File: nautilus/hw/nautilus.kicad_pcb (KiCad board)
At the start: 4 copper layers, 54.8 x 54 mm, 107 parts, among them IC1 DRV8353SRTAR, IC2 STM32G474CEU6, IC3 MAX15062AATA+T, J1 XT30XT30PW_MALE, J2 Conn_01x02_Pin, J3 Conn_01x02_Pin, M1 PAD24AWG_PAD, M2 PAD24AWG_PAD, M3 PAD24AWG_PAD, U2 CSD88599Q5DCT, U3 CSD88599Q5DCT, U4 AS5147, U5 CSD88599Q5DCT

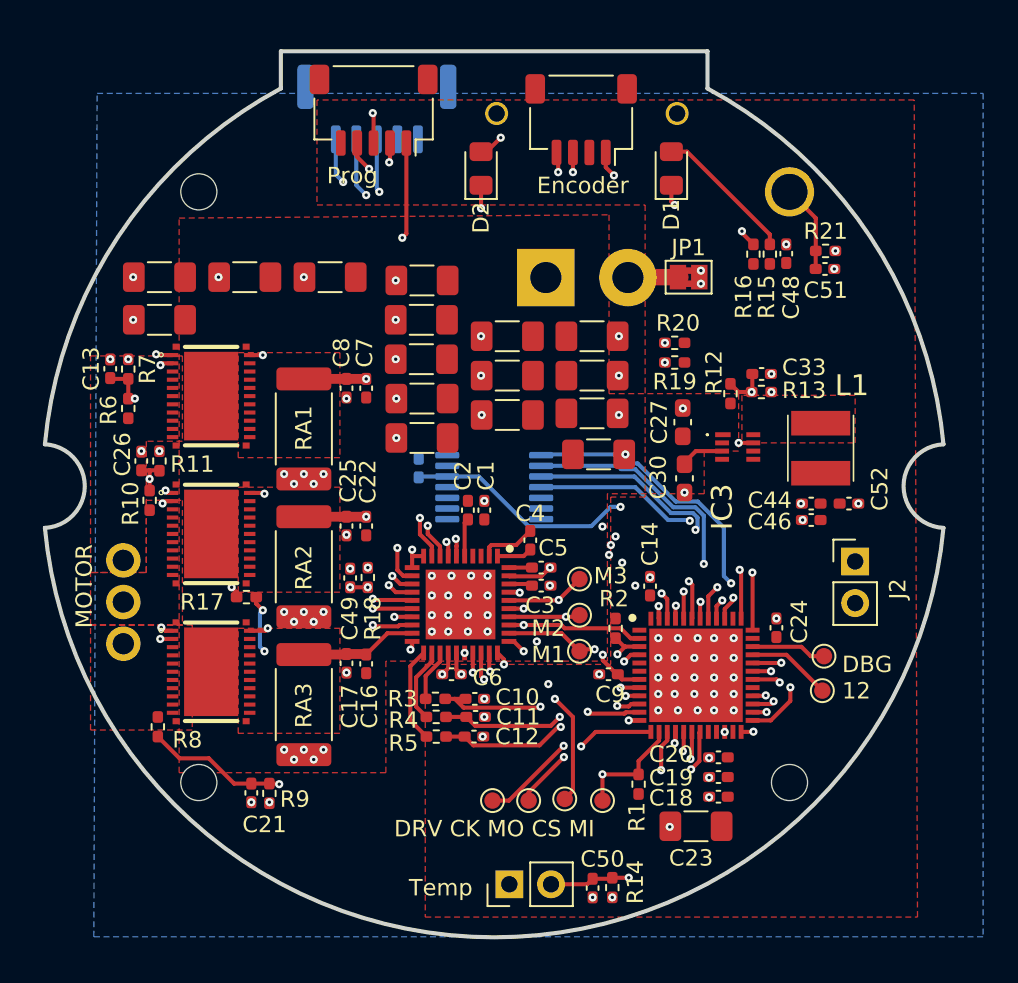
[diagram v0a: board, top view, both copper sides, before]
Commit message: Cleanup PCB before order
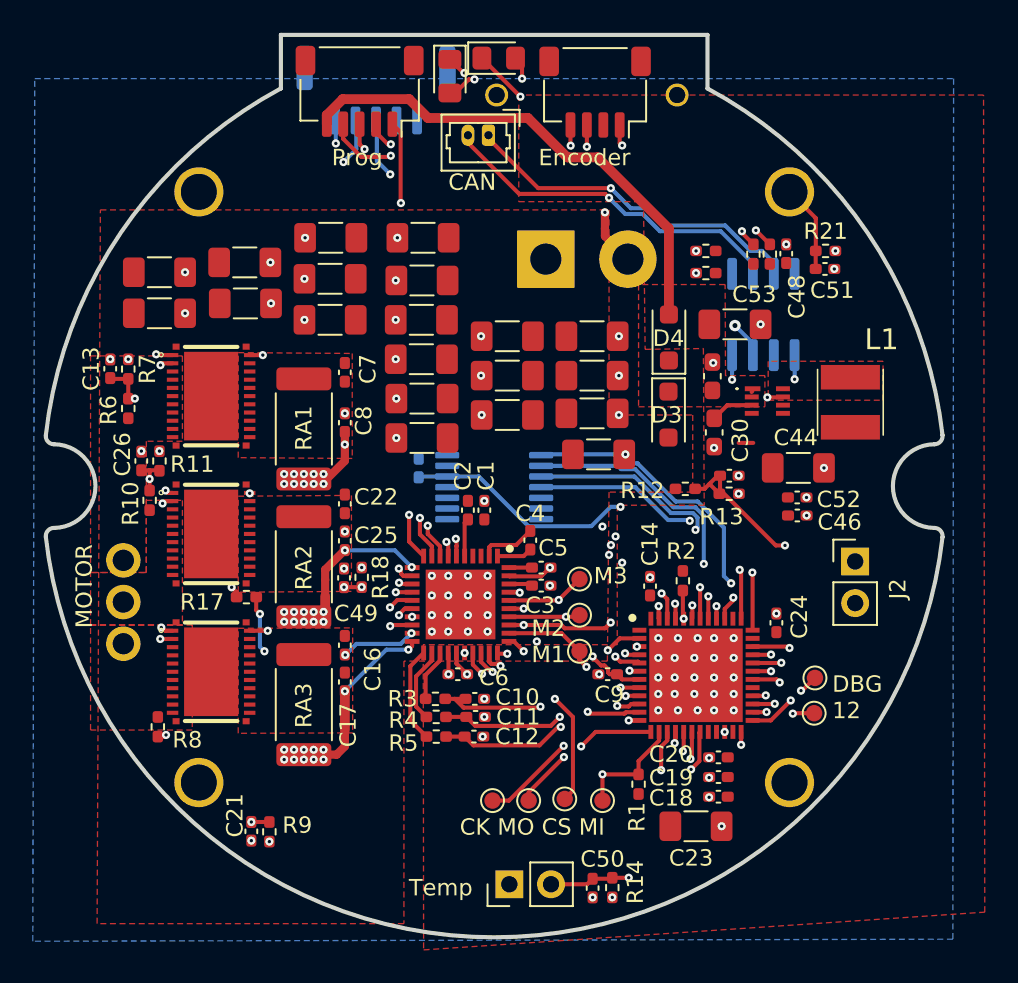
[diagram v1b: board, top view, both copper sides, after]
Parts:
- removed JP1: SolderJumper_2_Bridged, Jumper:SolderJumper-2_P1.3mm_Bridged2Bar_Pad1.0x1.5mm
- added C53: 10uF 50V, Capacitor_SMD:C_1206_3216Metric_Pad1.33x1.80mm_HandSolder, F.Cu at (160.7, 72.5)
- added C54: 10uF, Capacitor_SMD:C_1206_3216Metric_Pad1.33x1.80mm_HandSolder, F.Cu at (130.8, 71.2)
- added C55: 10uF, Capacitor_SMD:C_1206_3216Metric_Pad1.33x1.80mm_HandSolder, F.Cu at (136.0, 72.2)
- added C56: 10uF, Capacitor_SMD:C_1206_3216Metric_Pad1.33x1.80mm_HandSolder, F.Cu at (141.7, 67.2)
- added C57: 10uF, Capacitor_SMD:C_1206_3216Metric_Pad1.33x1.80mm_HandSolder, F.Cu at (136.0, 67.2)
- added D3: D_Schottky, Diode_SMD:D_SOD-123F, F.Cu at (156.6, 78.0)
- added D4: D_Schottky, Diode_SMD:D_SOD-123F, F.Cu at (156.7, 73.3)
- added J4: Conn_01x02_Pin, Connector_Molex:Molex_PicoBlade_53047-0210_1x02_P1.25mm_Vertical, F.Cu at (145.7, 61.0)
- added NT1: NetTie_2, NetTie:NetTie-2_SMD_Pad0.5mm, F.Cu at (136.9, 97.7)
- added NT2: NetTie_2, NetTie:NetTie-2_SMD_Pad0.5mm, F.Cu at (136.9, 80.3)
- added NT3: NetTie_2, NetTie:NetTie-2_SMD_Pad0.5mm, F.Cu at (135.7, 88.5)
- added NT4: NetTie_2, NetTie:NetTie-2_SMD_Pad0.5mm, F.Cu at (152.8, 66.2)
- added U7: SN65HVD232, Package_SO:SOIC-8_3.9x4.9mm_P1.27mm, B.Cu at (162.4, 71.9)
- C23: value 10uF -> 10uF 50V
- C28, C29, C31, C32, C34, C35, C36, C37, C38, C39, C40, C41, C42, C43, C45, C47: value 10uF 50V -> 10uF
- C44: value 10uF -> 10uF 50V; footprint Capacitor_SMD:C_0402_1005Metric_Pad0.74x0.62mm_HandSolder -> Capacitor_SMD:C_1206_3216Metric_Pad1.33x1.80mm_HandSolder
- C49: value 0.1uF -> 10nF
- H1, H3, H4: footprint MountingHole:MountingHole_2.2mm_M2_ISO7380 -> nautilus:MountingHole-Plated
- R10, R6, R8: value 100k -> 100k 1%
- R11, R7, R9: value 5.1k -> 4.7k 1%
- RA1, RA2, RA3: value 1.0mOhm 1% 2W -> 0.5mOhm 1% 2W
- moved D1 12.5 mm to (146.3, 56.2), turned to 0 degrees
- moved C33 6.50 mm to (160.3, 81.7)
- moved R13 6.50 mm to (160.3, 82.8)
- moved R12 6.42 mm to (157.7, 82.5), turned to 180 degrees
- moved D2 5.94 mm to (143.3, 57.4), turned to -90 degrees
- moved R20 5.91 mm to (158.9, 68.0)
- moved R19 5.77 mm to (158.9, 69.3)
- moved R2 5.02 mm to (157.5, 88.1)
- moved L1 3.33 mm to (167.7, 77.2)
- moved C27 3.33 mm to (159.3, 75.6)
- moved C30 3.33 mm to (159.4, 79.1)
- moved IC3 3.33 mm to (162.7, 77.2)
- moved C52 3.18 mm to (164.5, 83.0)
- moved C21 2.34 mm to (131.2, 103.4)
- moved R9 2.34 mm to (132.3, 103.4)
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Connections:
- net /FCUR1 renamed Net-(IC2-PB0)
- net /FCUR2 renamed Net-(IC2-PB1)
- net /FCUR3 renamed Net-(IC2-PB2)
- C17 pad 2: GNDPWR -> /SXC_N
- C23 pad 1: GNDS -> +3.3V
- C23 pad 2: +3.3V -> GNDS
- C25 pad 2: GNDPWR -> /SXB_N
- C27 pad 1: V+ -> Net-(D3-K)
- C8 pad 2: GNDPWR -> /SXA_N
- DEBUG1 pad 5: +3.3V -> +5V
- IC1 pad 10: GNDPWR -> /SXA_N
- IC1 pad 11: GNDPWR -> /SXB_N
- IC1 pad 20: GNDPWR -> /SXC_N
- IC2 pad 2: /MOTOR_HIZ -> /DRV8323_CS
- IC2 pad 3: /MOTOR_FAULT -> /DEBUG1
- IC2 pad 33: /DEBUG2 -> /CAN_RX
- IC2 pad 34: /DEBUG1 -> /CAN_TX
- IC2 pad 4: /DRV8323_CS -> /DEBUG2
- IC2 pad 44: /LED1 -> /MOTOR_FAULT
- IC2 pad 45: /LED2 -> /MOTOR_HIZ
- IC2 pad 5: unconnected-(IC2-PF0-OSC_IN-Pad5) -> /LED1
- IC2 pad 6: unconnected-(IC2-PF1-OSC_OUT-Pad6) -> /LED2
- IC3 pad 1: V+ -> Net-(D3-K)
- IC3 pad 2: V+ -> Net-(D3-K)
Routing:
- net +5V: track 0.00 -> 30.3 mm
- net /CAN_TX: track 0.00 -> 22.1 mm, vias 0 -> 2
- net /LED1: track 27.4 -> 49.4 mm
- net Net-(J4-Pin_1): track 0.00 -> 21.1 mm, vias 0 -> 1
- net /CAN_RX: track 0.00 -> 21.0 mm, vias 0 -> 2
- net Net-(J4-Pin_2): track 0.00 -> 20.8 mm, vias 0 -> 1
- net Net-(D1-A): track 8.69 -> 20.1 mm, vias 0 -> 2
- net /LED2: track 34.0 -> 44.7 mm, vias 3 -> 2
- net /SXA_N: track 0.00 -> 9.62 mm, vias 0 -> 2
- net /DEBUG2: track 5.16 -> 14.6 mm, vias 0 -> 2
- net /SXC_N: track 0.00 -> 7.88 mm, vias 0 -> 2
- net /DEBUG1: track 4.59 -> 12.3 mm, vias 0 -> 2
- net /SXB_N: track 0.00 -> 6.76 mm, vias 0 -> 2
- net /SXA_P: track 16.3 -> 10.9 mm
- net /VBAT_SENSE: track 25.2 -> 21.5 mm
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- added copper zone on F.Cu, net Net-(D3-K)
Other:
- board size 54.8 x 54 mm -> 54.7 x 55 mm
- board text added: "CAN"
- board text added: "CK MO CS MI"
- board text removed: "DRV CK MO CS MI"
